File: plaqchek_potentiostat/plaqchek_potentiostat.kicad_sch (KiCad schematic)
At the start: 33 parts, among them J1 Conn_01x03, J2 Conn_01x03, SW1 SW_DPDT_x2, U1 Opamp_Dual, U2 L78L05_SOT89, U3 Opamp_Dual, U4 Opamp_Dual, U5 TPS7A2050PDBVR, U8 MC79M05_TO252

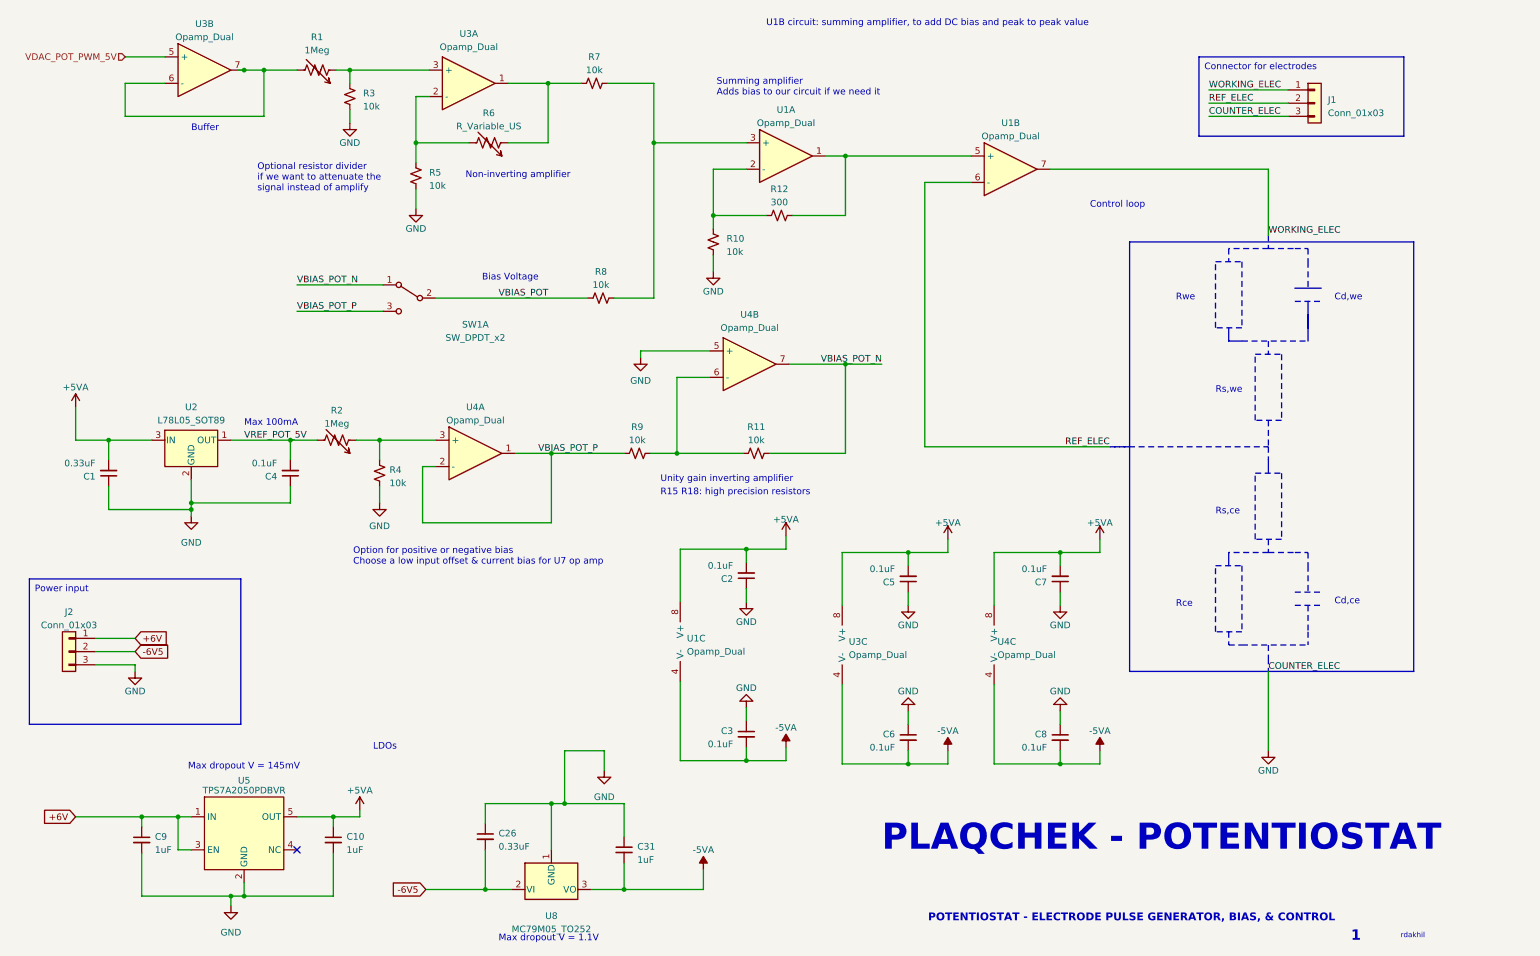
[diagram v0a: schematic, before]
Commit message: finish schematic
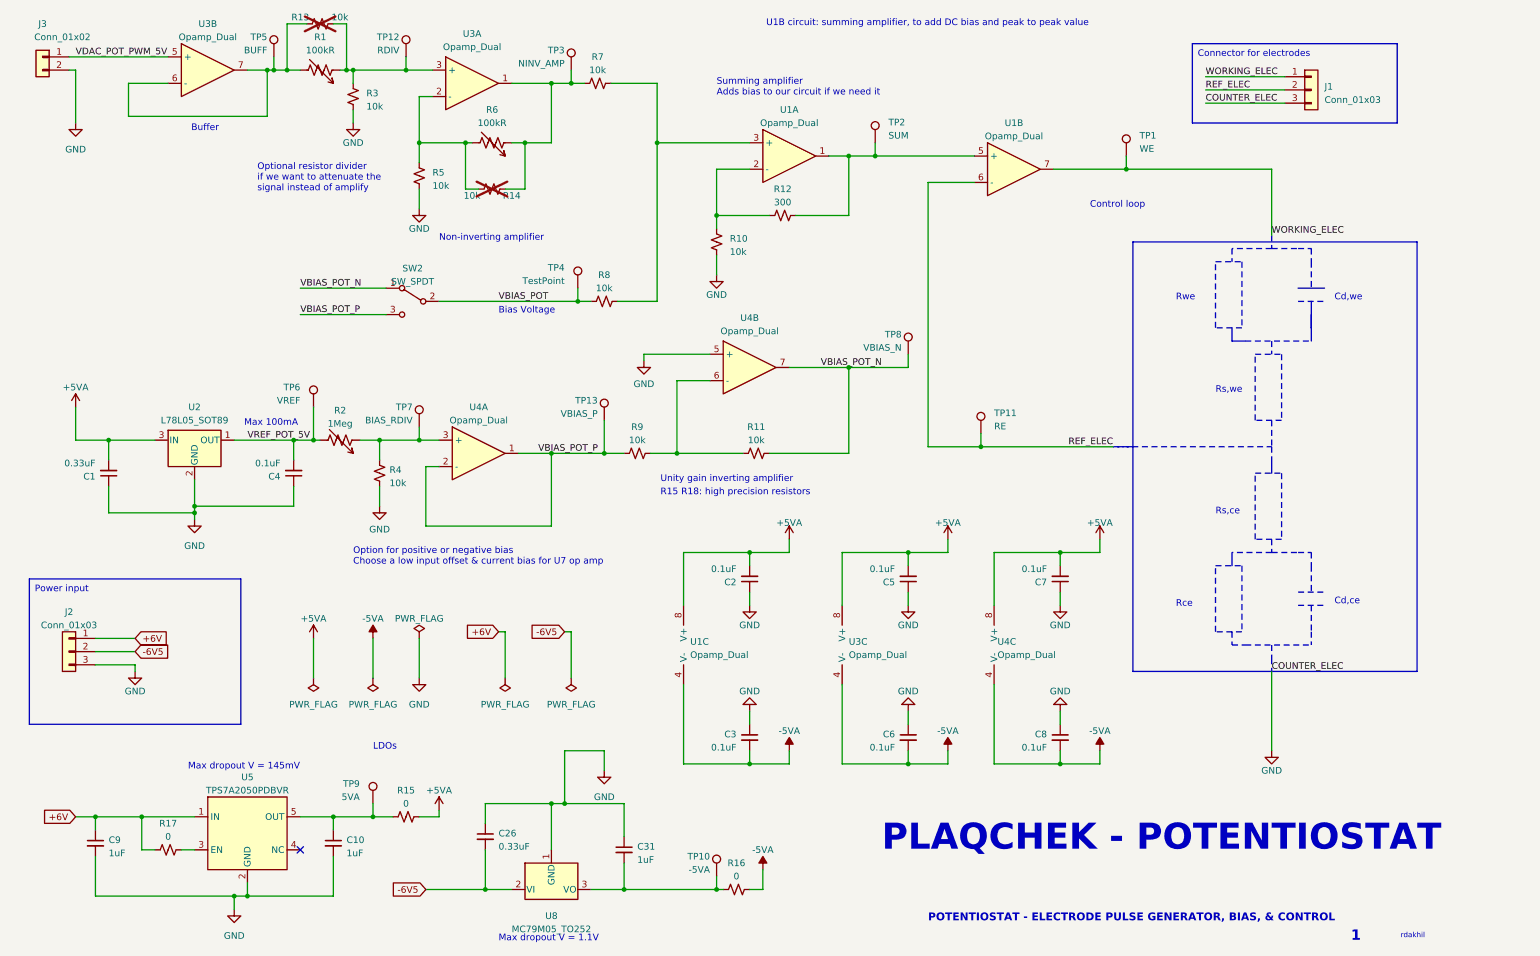
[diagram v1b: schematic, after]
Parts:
- removed SW1: SW_DPDT_x2, symbol Switch:SW_DPDT_x2
- removed U5: TPS7A2050PDBVR, symbol plaqchek_mlb:TPS7A2050PDBVR
- added J3: Conn_01x02, symbol Connector_Generic:Conn_01x02
- added R13, R14: 10k, symbol Device:R_Small_US
- added R15, R16, R17: 0, symbol Device:R_Small_US
- added SW2: SW_SPDT, symbol Switch:SW_SPDT
- added TP1: WE, symbol Connector:TestPoint
- added TP10: -5VA, symbol Connector:TestPoint
- added TP11: RE, symbol Connector:TestPoint
- added TP12: RDIV, symbol Connector:TestPoint
- added TP13: VBIAS_P, symbol Connector:TestPoint
- added TP2: SUM, symbol Connector:TestPoint
- added TP3: NINV_AMP, symbol Connector:TestPoint
- added TP4: TestPoint, symbol Connector:TestPoint
- added TP5: BUFF, symbol Connector:TestPoint
- added TP6: VREF, symbol Connector:TestPoint
- added TP7: BIAS_RDIV, symbol Connector:TestPoint
- added TP8: VBIAS_N, symbol Connector:TestPoint
- added TP9: 5VA, symbol Connector:TestPoint
- added U5: TPS7A2050PDBVR, symbol plaqchek:TPS7A2050PDBVR
- R1: value 1Meg -> 100kR
- R6: value R_Variable_US -> 100kR
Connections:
- net +5VA: now also R15.1; no longer C10.1
- net +6V: now also R17.2, U5.1 (IN)
- net -5VA: now also R16.1; no longer C31.2, U8.3 (VO)
- net GND: now also J3.2 (Pin_2), U5.2 (GND)
- net REF_ELEC: now also TP11.1
- net VBIAS_POT: now also SW2.2 (B), TP4.1
- net VBIAS_POT_N: now also SW2.1 (A), TP8.1
- net VBIAS_POT_P: now also SW2.3 (C), TP13.1
- net VDAC_POT_PWM_5V: now also J3.1 (Pin_1)
- net VREF_POT_5V: now also TP6.1
- net WORKING_ELEC: now also TP1.1
- net at R2.1, R4.2, U4.3 (+): now also TP7.1
- net at R12.2, U1.1, U1.5 (+): now also TP2.1
- net at R1.2, U3.6 (-), U3.7: now also R13.2, TP5.1
- net at R1.1, R3.2, U3.3 (+): now also R13.1, TP12.1
- net at R6.1, R7.1, U3.1: now also R14.2, TP3.1
- net at R5.2, R6.2, U3.2 (-): now also R14.1
- new net: R17.1, U5.3 (EN)
- new net: C31.2, R16.2, TP10.1, U8.3 (VO)
- new net: C10.1, R15.2, TP9.1, U5.5 (OUT)
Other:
- moved on the sheet: C10, C2, C3, C4, C9, J1, R1, R10, R12, R2, R3, R5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

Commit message: finish main logic board PCB routing
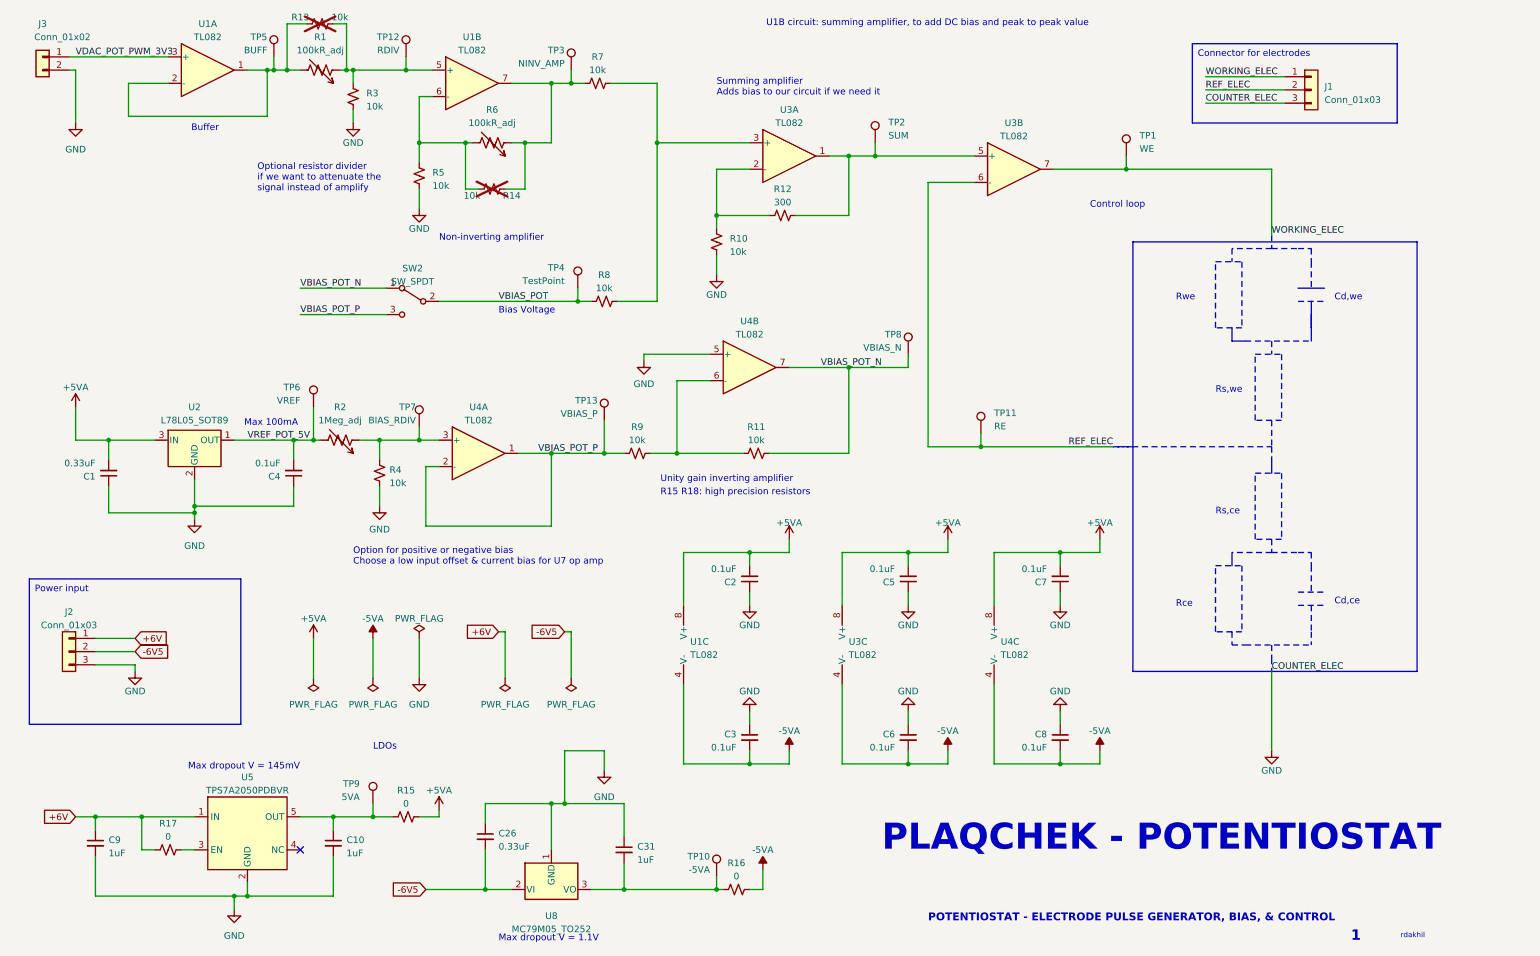
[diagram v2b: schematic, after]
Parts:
- removed U1, U3, U4: Opamp_Dual, symbol Device:Opamp_Dual
- added U1, U3, U4: TL082, Package_TO_SOT_SMD:TSOT-23-8_HandSoldering, symbol Amplifier_Operational:TL082
- C1, C10, C2, C26, C3, C31, C4, C5, C6, C7, C8, C9: footprint (none) -> Capacitor_SMD:C_0603_1608Metric_Pad1.08x0.95mm_HandSolder
- J1, J2: footprint (none) -> Connector_PinHeader_2.54mm:PinHeader_1x03_P2.54mm_Vertical
- J3: footprint (none) -> Connector_PinHeader_2.54mm:PinHeader_1x02_P2.54mm_Vertical
- R1, R6: value 100kR -> 100kR_adj
- R10, R11, R12, R13, R14, R15, R16, R17, R3, R4, R5, R7, R8, R9: footprint (none) -> Resistor_SMD:R_0603_1608Metric_Pad0.98x0.95mm_HandSolder
- R2: value 1Meg -> 1Meg_adj
- U5: footprint (none) -> Package_TO_SOT_SMD:SOT-23-5_HandSoldering
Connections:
- net +5VA: now also U1.8 (V+), U3.8 (V+), U4.8 (V+)
- net -5VA: now also U1.4 (V-), U3.4 (V-), U4.4 (V-)
- net GND: now also U4.5 (+)
- net REF_ELEC: now also U3.6 (-)
- net VBIAS_POT_N: now also U4.7
- net VBIAS_POT_P: now also U4.1, U4.2 (-)
- net WORKING_ELEC: now also U3.7
- net at R2.1, R4.2, TP7.1: now also U4.3 (+)
- net at R1.2, R13.2, TP5.1: now also U1.1, U1.2 (-)
- net at R12.2, TP2.1: now also U3.1, U3.5 (+)
- net at R10.2, R12.1: now also U3.2 (-)
- net at R7.2, R8.2: now also U3.3 (+)
- net at R1.1, R13.1, R3.2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: now also U1.5 (+)
- net at R11.2, R9.1: now also U4.6 (-)
- net at R14.2, R6.1, R7.1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: now also U1.7
- net at R14.1, R5.2, R6.2: now also U1.6 (-)
- net VDAC_POT_PWM_5V renamed VDAC_POT_PWM_3V3
- net VDAC_POT_PWM_3V3: now also U1.3 (+)
